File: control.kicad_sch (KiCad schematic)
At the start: 40 parts, among them J4 Conn_01x05_Pin, J5 Conn_01x03_Pin, J6 Conn_01x03_Pin, Q2 AO3400, Q3 DTC143Z, Q4 DMG1012T, SW2 SW_Push, SW3 SW_SPDT, U6 STM32G031G8Ux

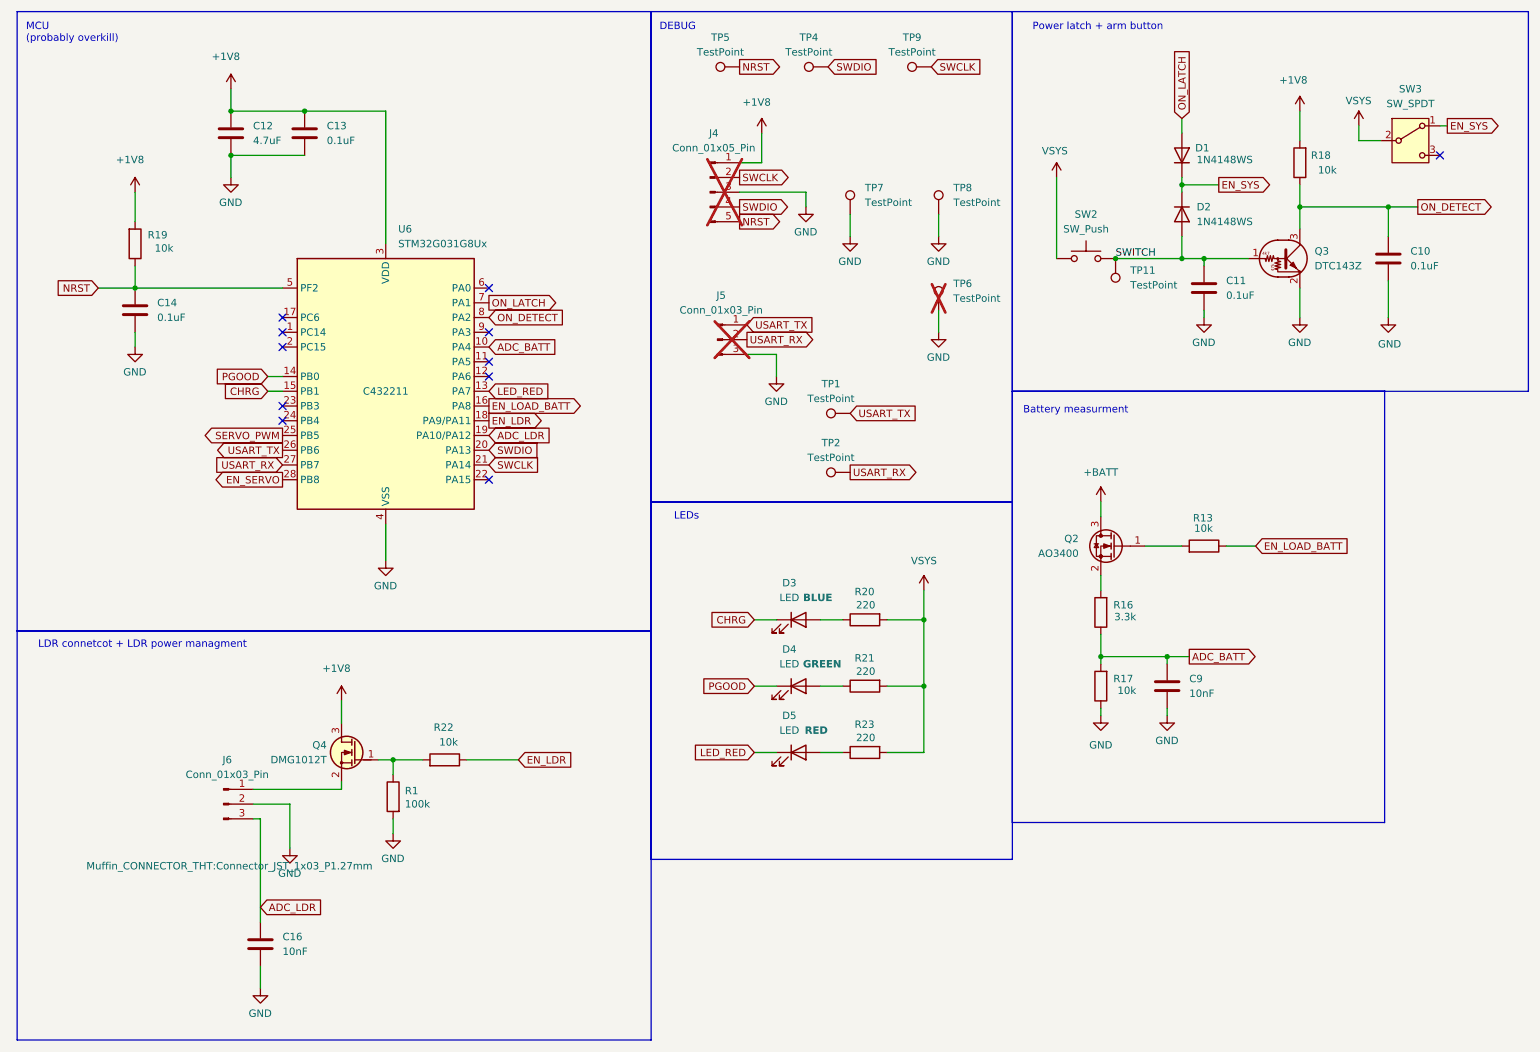
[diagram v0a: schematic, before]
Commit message: Expanded documentation
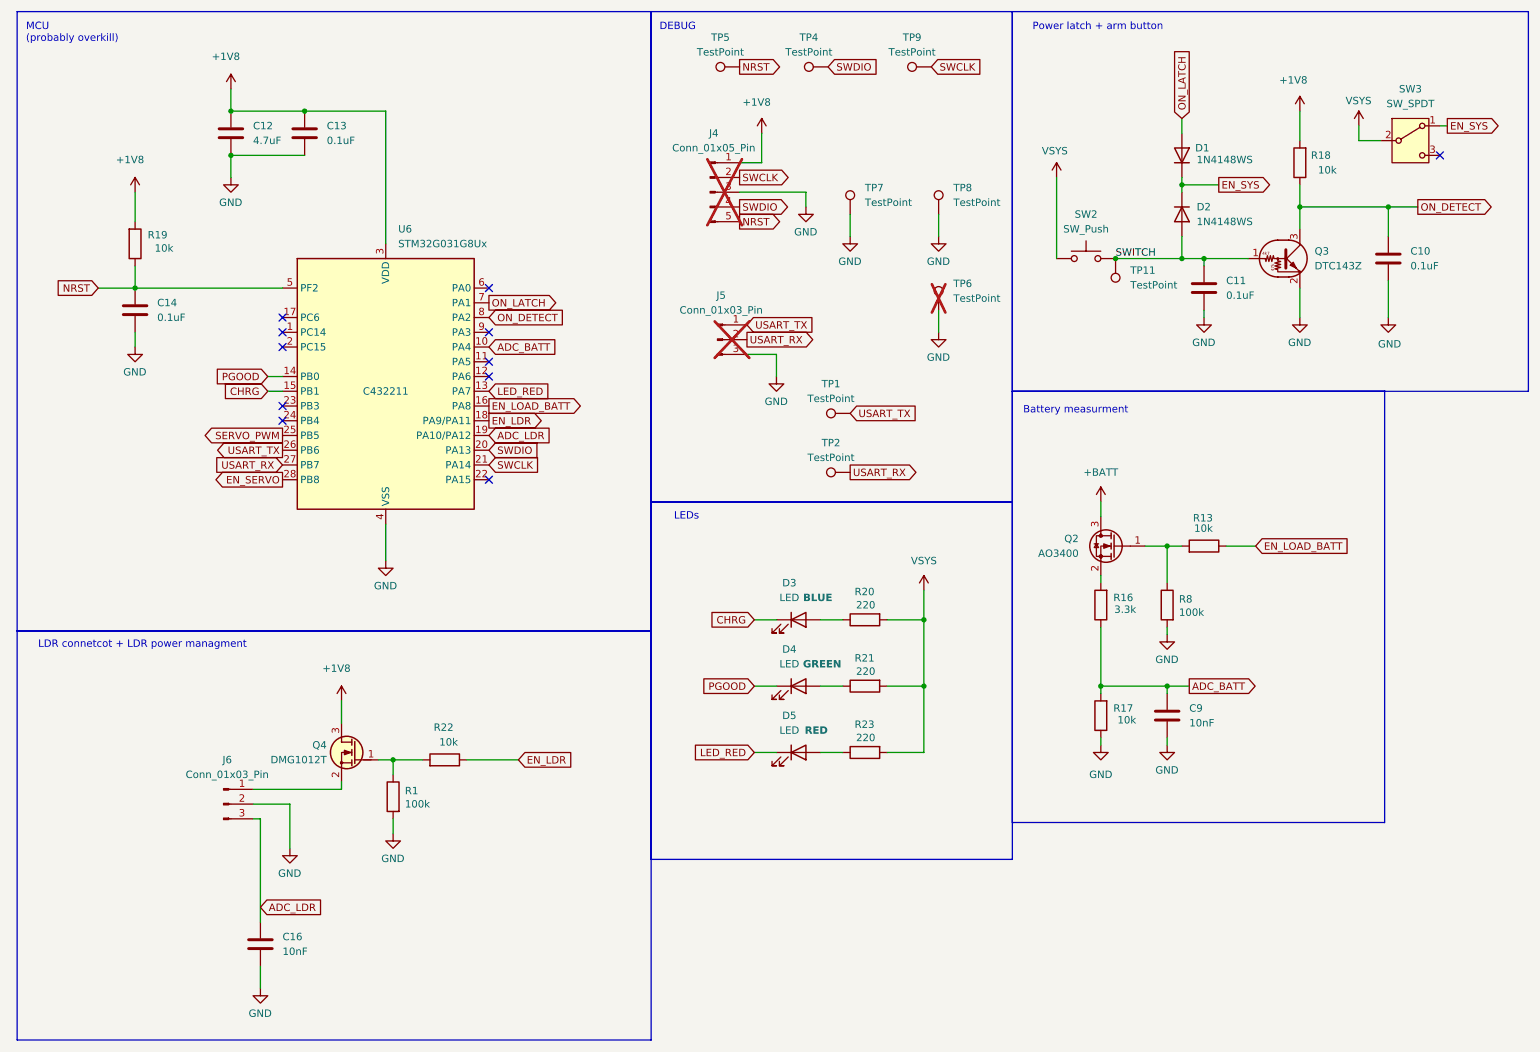
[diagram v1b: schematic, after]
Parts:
- added R8: 100k, Resistor_SMD:R_0603_1608Metric, symbol Device:R
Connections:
- net GND: now also R8.2
- net at Q2.1 (G), R13.2: now also R8.1
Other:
- moved on the sheet: C9, R16, R17
